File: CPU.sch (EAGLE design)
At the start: 3 parts, among them IC1 Z80CPU

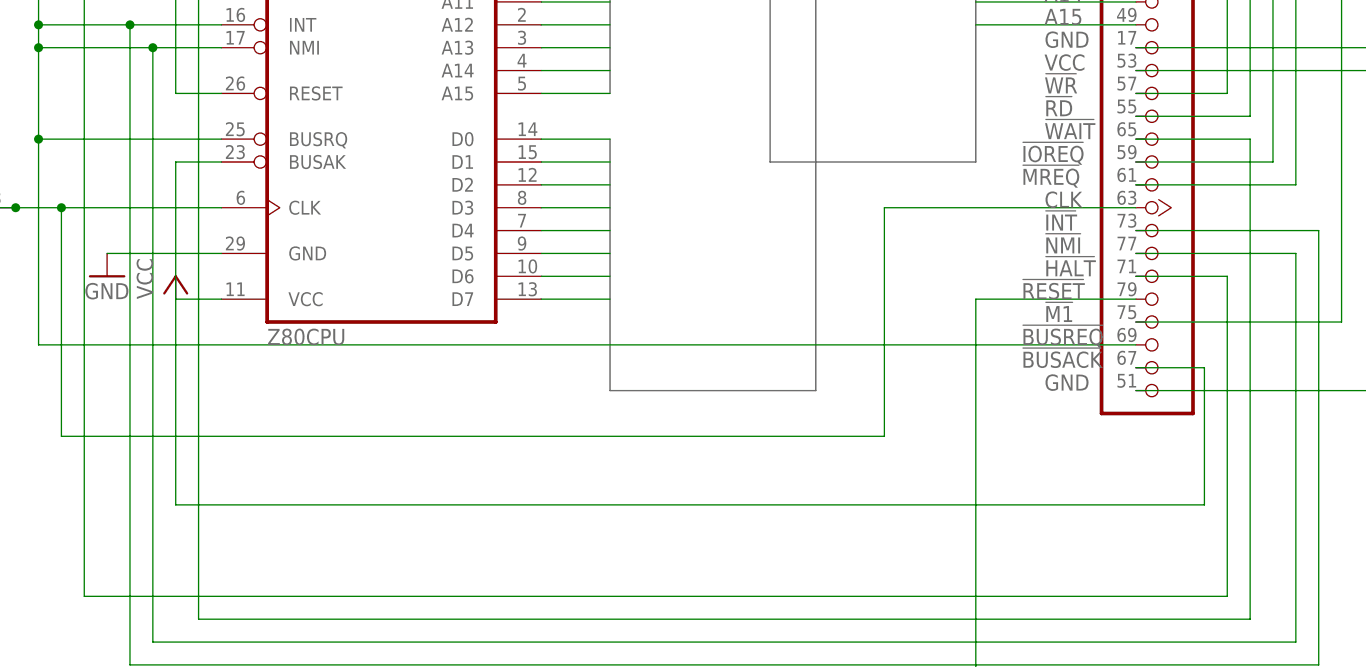
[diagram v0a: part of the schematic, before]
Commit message: Finish Modularization
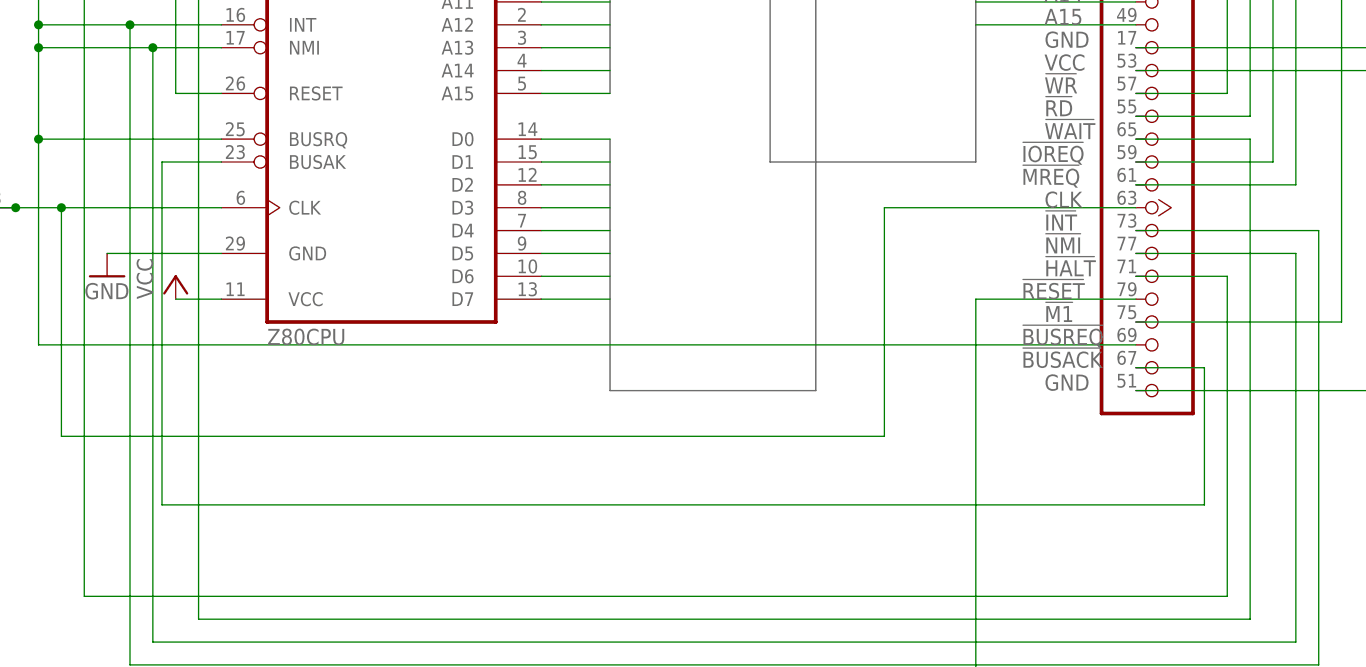
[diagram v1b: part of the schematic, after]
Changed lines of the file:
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@@
 <wire x1="96.52" y1="20.32" x2="104.14" y2="20.32" width="0.1524" layer="91"/>
 <wire x1="104.14" y1="20.32" x2="104.14" y2="5.08" width="0.1524" layer="91"/>
-<wire x1="104.14" y1="5.08" x2="-10.16" y2="5.08" width="0.1524" layer="91"/>
-<wire x1="-10.16" y1="5.08" x2="-10.16" y2="43.18" width="0.1524" layer="91"/>
+<wire x1="104.14" y1="5.08" x2="-11.684" y2="5.08" width="0.1524" layer="91"/>
+<wire x1="-11.684" y1="5.08" x2="-11.684" y2="43.18" width="0.1524" layer="91"/>
 <pinref part="IC1" gate="1" pin="BUSAK"/>
-<wire x1="-10.16" y1="43.18" x2="-5.08" y2="43.18" width="0.1524" layer="91"/>
+<wire x1="-11.684" y1="43.18" x2="-5.08" y2="43.18" width="0.1524" layer="91"/>
 </segment>
 </net>
@@
 </sheet>
 </sheets>
-<errors>
-</errors>
 </schematic>
 </drawing>
